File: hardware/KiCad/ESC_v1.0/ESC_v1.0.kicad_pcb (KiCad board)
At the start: 6 copper layers, 56.6 x 43.2 mm, 105 parts, among them J1 Conn_ARM_SWD_TagConnect_TC203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, J3 USB4105-GF-A, Q3 CSD18540Q5B, Q4 CSD18540Q5B, U2 LM5160A, U3 TPS7B92033, U4 STM32G484CEU6, U5 2EDL8024, U8 TPD2EUSB30A, X2 16MHz

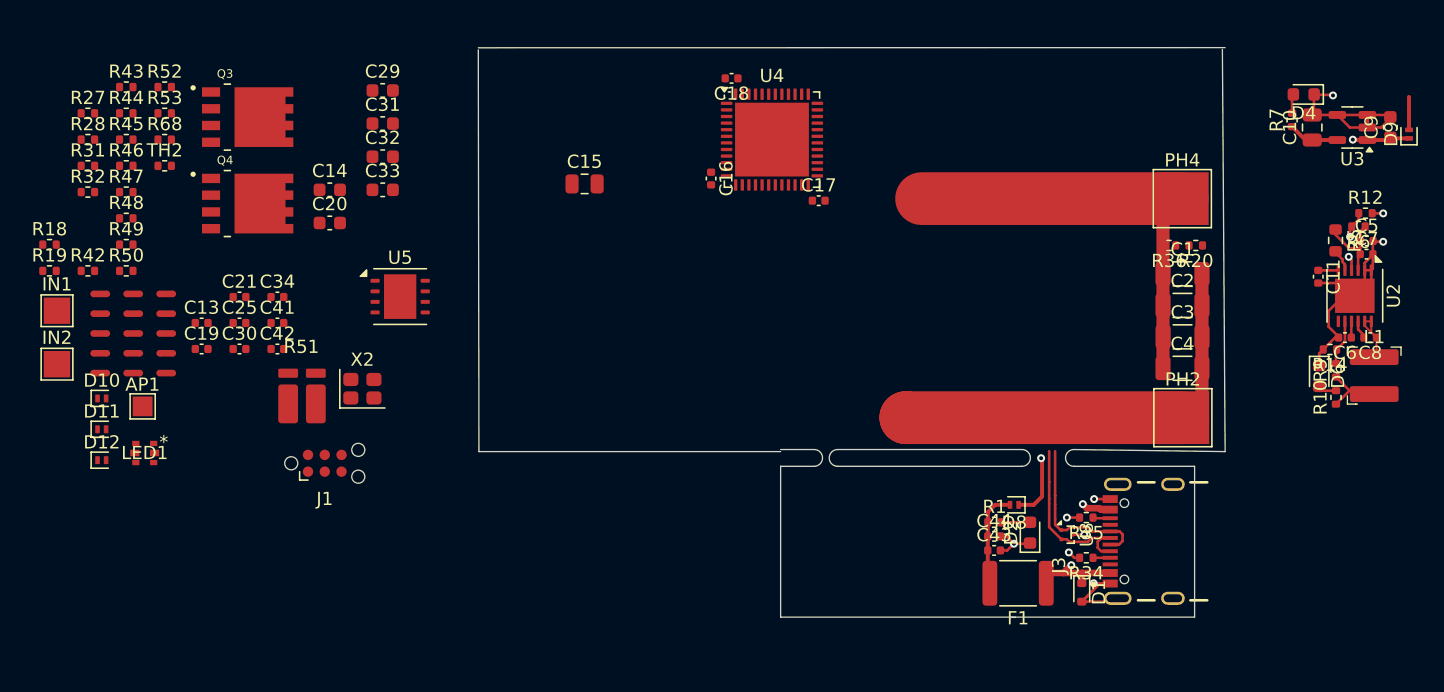
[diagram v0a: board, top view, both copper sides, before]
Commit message: Major board update
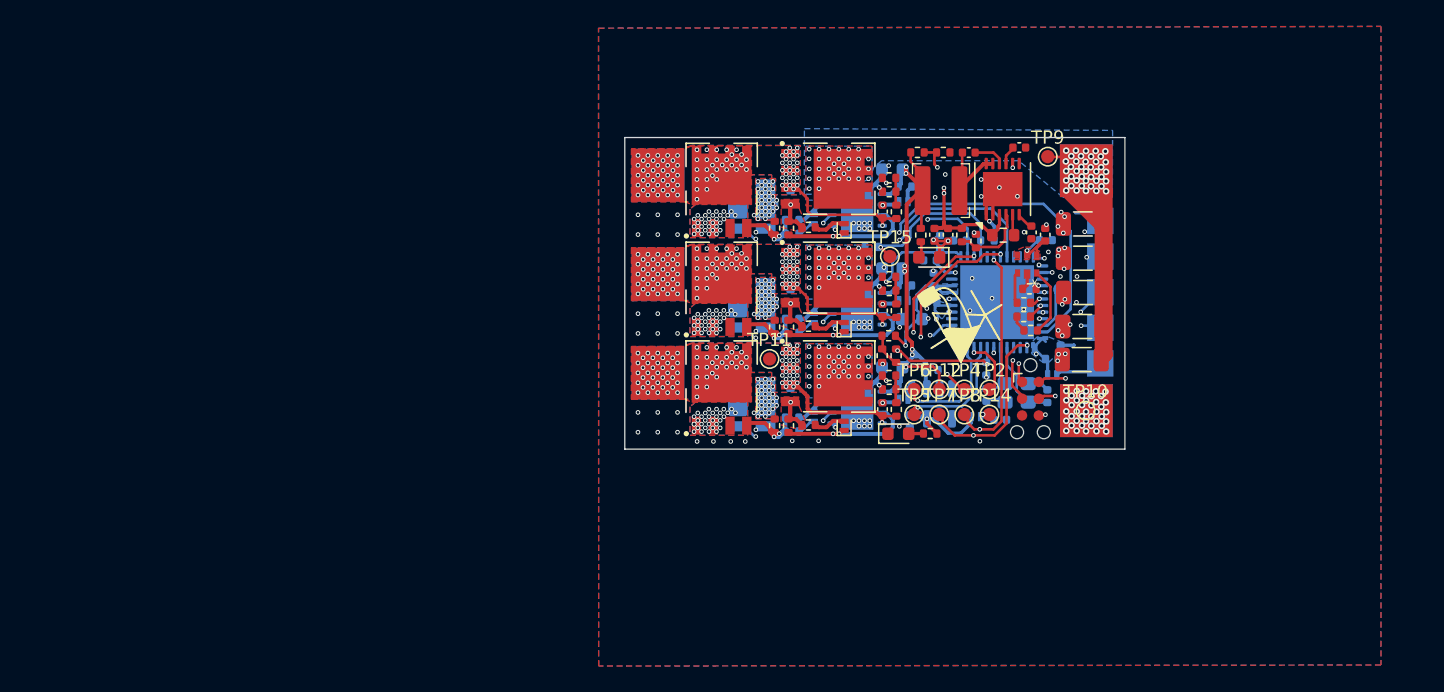
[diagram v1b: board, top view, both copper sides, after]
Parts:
- removed AP1: ActionPad, TestPoint:TestPoint_Pad_1.5x1.5mm
- removed C10: 4.7u, Capacitor_SMD:C_0805_2012Metric
- removed the C14 at (58.5, 45.0)
- removed the C16 at (87.4, 44.1)
- removed the C17 at (95.6, 45.8)
- removed the C4 at (123.2, 58.5)
- removed C41, C42: 10p, Capacitor_SMD:C_0402_1005Metric
- removed C43: 1u, Capacitor_SMD:C_0402_1005Metric
- removed C44: 100n, Capacitor_SMD:C_0402_1005Metric
- removed the C5 at (137.1, 48.8)
- removed C9: 1u, Capacitor_SMD:C_0603_1608Metric
- removed the D1 at (115.5, 75.5)
- removed F1: Polyfuse, Resistor_SMD:R_1812_4532Metric
- removed IN1, IN2: ~, TestPoint:TestPoint_Pad_2.0x2.0mm
- removed NT1, NT10, NT11, NT12, NT13, NT14, NT15, NT2, NT3, NT4, NT5, NT6, NT7, NT8, NT9: NetTie_2, NetTie:NetTie-2_SMD_Pad0.5mm
- removed PH2, PH4: ~, TestPoint:TestPoint_Pad_4.0x4.0mm
- removed the R5 at (134.8, 48.8)
- removed R51: 0.5m, ESC-FootprintLib:Kelvin Shunt 1216 (3038)
- removed R52: 33, Resistor_SMD:R_0402_1005Metric
- removed R53: 10k, Resistor_SMD:R_0402_1005Metric
- removed the R6 at (136.5, 47.7)
- removed R68: 0R, Resistor_SMD:R_0402_1005Metric
- removed TH2: Thermistor_NTC, Resistor_SMD:R_0402_1005Metric
- removed U8: TPD2EUSB30A, Package_TO_SOT_SMD:Texas_DRT-3
- removed X2: 16MHz, Crystal:Crystal_SMD_2520-4Pin_2.5x2.0mm
- added C1: 1u, Capacitor_SMD:C_0402_1005Metric, B.Cu at (102.5, 62.5)
- added C11: 100n, Capacitor_SMD:C_0402_1005Metric, B.Cu at (113.9, 56.3)
- added C12: 1u, Capacitor_SMD:C_0402_1005Metric, F.Cu at (104.4, 48.4)
- added C2: 100n, Capacitor_SMD:C_0402_1005Metric, B.Cu at (104.0, 50.3)
- added C23: 1u, Capacitor_SMD:C_0402_1005Metric, B.Cu at (104.2, 58.6)
- added C24: 100n, Capacitor_SMD:C_0402_1005Metric, B.Cu at (108.3, 58.5)
- added C26: 220n, Capacitor_SMD:C_0402_1005Metric, F.Cu at (100.4, 46.6)
- added C27: 1u, Capacitor_SMD:C_0603_1608Metric, B.Cu at (101.2, 43.4)
- added C28: 100n, Capacitor_SMD:C_0402_1005Metric, B.Cu at (106.3, 48.8)
- added C37: 100n, Capacitor_SMD:C_0402_1005Metric, B.Cu at (112.8, 48.8)
- added C6: 2.2u, Capacitor_SMD:C_1206_3216Metric, F.Cu at (115.6, 55.3)
- added C8: 2.2u, Capacitor_SMD:C_1206_3216Metric, F.Cu at (115.5, 57.8)
- added D13: RB161QS-40T18R, ESC-FootprintLib:Rohm_SMD1006, B.Cu at (95.2, 62.2)
- added D14: RB161QS-40T18R, ESC-FootprintLib:Rohm_SMD1006, B.Cu at (113.3, 59.0)
- added D5: RB161QS-40T18R, ESC-FootprintLib:Rohm_SMD1006, B.Cu at (102.0, 45.9)
- added D6: RB161QS-40T18R, ESC-FootprintLib:Rohm_SMD1006, F.Cu at (97.5, 47.9)
- added D7: RB161QS-40T18R, ESC-FootprintLib:Rohm_SMD1006, B.Cu at (95.2, 47.2)
- added J10: Conn_01x01, TestPoint:TestPoint_Pad_2.0x2.0mm, B.Cu at (116.9, 58.1)
- added J11: JTAG_TC2030, Connector:Tag-Connect_TC2030-IDC-NL_2x03_P1.27mm_Vertical, F.Cu at (111.6, 60.8)
- added J2: Conn_01x01, ESC-FootprintLib:Phase4x4, F.Cu at (115.9, 61.7)
- added J4: Conn_01x01, TestPoint:TestPoint_Pad_2.0x2.0mm, B.Cu at (116.9, 52.7)
- added J5: Conn_01x01, TestPoint:TestPoint_Pad_2.0x2.0mm, B.Cu at (116.9, 47.3)
- added J6: Conn_01x01, TestPoint:TestPoint_Pad_2.0x2.0mm, B.Cu at (116.9, 50.0)
- added J7: Conn_01x01, ESC-FootprintLib:Phase4x4, F.Cu at (83.4, 43.9)
- added J8: Conn_01x01, ESC-FootprintLib:Phase4x4, F.Cu at (83.4, 51.4)
- added J9: Conn_01x01, ESC-FootprintLib:Phase4x4, F.Cu at (83.4, 58.8)
- added Q1: CSD18540Q5B, ESC-FootprintLib:TRANS_CSD18540Q5B, F.Cu at (96.2, 44.1)
- added Q2: CSD18540Q5B, ESC-FootprintLib:TRANS_CSD18540Q5B, F.Cu at (88.2, 45.1)
- added Q5: CSD18540Q5B, ESC-FootprintLib:TRANS_CSD18540Q5B, F.Cu at (96.2, 59.1)
- added Q6: CSD18540Q5B, ESC-FootprintLib:TRANS_CSD18540Q5B, F.Cu at (88.2, 60.1)
- added R11: 100, Resistor_SMD:R_0402_1005Metric, F.Cu at (104.0, 63.4)
- added R13: 33, Resistor_SMD:R_0402_1005Metric, F.Cu at (101.5, 57.5)
- added R14: 100, Resistor_SMD:R_0402_1005Metric, F.Cu at (111.1, 54.6)
- added R15: 100, Resistor_SMD:R_0402_1005Metric, F.Cu at (111.7, 55.6)
- added R16: 100, Resistor_SMD:R_0402_1005Metric, F.Cu at (111.6, 52.5)
- added R17: 100, Resistor_SMD:R_0402_1005Metric, F.Cu at (111.1, 53.5)
- added R2: 10k, Resistor_SMD:R_0402_1005Metric, B.Cu at (108.4, 48.8)
- added R21: 10k, Resistor_SMD:R_0402_1005Metric, B.Cu at (93.5, 45.6)
- added R22: 3.3, Resistor_SMD:R_0402_1005Metric, B.Cu at (93.6, 47.2)
- added R23: 10, Resistor_SMD:R_0402_1005Metric, B.Cu at (93.6, 48.3)
- added R24: 10k, Resistor_SMD:R_0402_1005Metric, F.Cu at (92.3, 47.9)
- added R25: 0.5m, ESC-FootprintLib:Kelvin Shunt 1216 (3038), B.Cu at (90.5, 46.3)
- added R26: 10k, Resistor_SMD:R_0402_1005Metric, F.Cu at (101.5, 46.6)
- added R29: 3.3, Resistor_SMD:R_0402_1005Metric, B.Cu at (102.1, 52.2)
- added R3: 120k, Resistor_SMD:R_0603_1608Metric, F.Cu at (109.6, 48.4)
- added R30: 10, Resistor_SMD:R_0402_1005Metric, F.Cu at (94.8, 55.3)
- added R33: 3.3, Resistor_SMD:R_0402_1005Metric, B.Cu at (93.6, 54.7)
- added R37: 10k, Resistor_SMD:R_0402_1005Metric, F.Cu at (101.5, 54.1)
- added R38: 33, Resistor_SMD:R_0402_1005Metric, F.Cu at (100.9, 51.6)
- added R39: 1k, Resistor_SMD:R_0402_1005Metric, F.Cu at (100.9, 52.6)
- added R4: 200k, Resistor_SMD:R_0402_1005Metric, F.Cu at (106.4, 48.4)
- added R40: 3.3, Resistor_SMD:R_0402_1005Metric, B.Cu at (102.1, 59.7)
- added R41: 10, Resistor_SMD:R_0402_1005Metric, F.Cu at (94.8, 62.8)
- added TH1: Thermistor_NTC, Resistor_SMD:R_0402_1005Metric, F.Cu at (100.4, 57.5)
- added TP1: TestPoint, TestPoint:TestPoint_Pad_D1.0mm, B.Cu at (113.9, 52.5)
- added TP10: TestPoint, TestPoint:TestPoint_Pad_D1.0mm, F.Cu at (115.8, 61.7)
- added TP11: TestPoint, TestPoint:TestPoint_Pad_D1.0mm, F.Cu at (91.9, 57.8)
- added TP12: TestPoint, TestPoint:TestPoint_Pad_D1.0mm, F.Cu at (104.7, 60.1)
- added TP14: TestPoint, TestPoint:TestPoint_Pad_D1.0mm, F.Cu at (108.5, 62.0)
- added TP15: TestPoint, TestPoint:TestPoint_Pad_D1.0mm, F.Cu at (101.0, 50.0)
- added TP2: TestPoint, TestPoint:TestPoint_Pad_D1.0mm, F.Cu at (108.5, 60.1)
- added TP4: TestPoint, TestPoint:TestPoint_Pad_D1.0mm, F.Cu at (106.6, 60.1)
- added TP5: TestPoint, TestPoint:TestPoint_Pad_D1.0mm, F.Cu at (102.8, 62.0)
- added TP6: TestPoint, TestPoint:TestPoint_Pad_D1.0mm, F.Cu at (102.8, 60.1)
- added TP7: TestPoint, TestPoint:TestPoint_Pad_D1.0mm, F.Cu at (104.7, 62.0)
- added TP8: TestPoint, TestPoint:TestPoint_Pad_D1.0mm, F.Cu at (106.6, 62.0)
- added TP9: TestPoint, TestPoint:TestPoint_Pad_D1.0mm, F.Cu at (113.0, 42.5)
- added U1: STM32G484CEU6, ESC-FootprintLib:QFN-48-1EP_7x7mm_P0.5mm_EP5.6x5.6mm, B.Cu at (109.1, 53.5)
- added U6: 2EDL8024, ESC-FootprintLib:2EDL8x2x_PG-VDSON-8-4, B.Cu at (98.5, 61.5)
- added X1: 16MHz, Crystal:Crystal_SMD_2520-4Pin_2.5x2.0mm, B.Cu at (110.6, 60.4)
- C13: value 10n -> 1u
- C15: value 4.7u -> 100n; footprint Capacitor_SMD:C_0805_2012Metric -> Capacitor_SMD:C_0402_1005Metric; moved to B.Cu
- C18: value 100n -> 10n; moved to B.Cu
- C19: value 100n -> 1u; footprint Capacitor_SMD:C_0402_1005Metric -> Capacitor_SMD:C_0603_1608Metric; moved to B.Cu
- C20: value 1u -> 10p; footprint Capacitor_SMD:C_0603_1608Metric -> Capacitor_SMD:C_0402_1005Metric; moved to B.Cu
- C21: value 100n -> 10p; moved to B.Cu
- C29, C32: value 100p -> 220n; footprint Capacitor_SMD:C_0603_1608Metric -> Capacitor_SMD:C_0402_1005Metric
- C30: value 220n -> 1u; footprint Capacitor_SMD:C_0402_1005Metric -> Capacitor_SMD:C_0603_1608Metric; moved to B.Cu
- C31: value 1u -> 100n; footprint Capacitor_SMD:C_0603_1608Metric -> Capacitor_SMD:C_0402_1005Metric; moved to B.Cu
- C33: value 100p -> 1u; moved to B.Cu
- C34, C7, D10, D11, D8, U3, U5: moved to B.Cu
- D2: value KT-0603W -> RB161QS-40T18R; footprint LED_SMD:LED_0603_1608Metric -> ESC-FootprintLib:Rohm_SMD1006; moved to B.Cu
- J1: value Conn_ARM_SWD_TagConnect_TC2030-NL -> Conn_01x01; footprint Connector:Tag-Connect_TC2030-IDC-NL_2x03_P1.27mm_Vertical -> ESC-FootprintLib:Phase4x4
- J3: value USB4105-GF-A -> Conn_01x01; footprint ESC-FootprintLib:GCT_USB4105-GF-A -> TestPoint:TestPoint_Pad_2.0x2.0mm; moved to B.Cu
- R1: value 1k -> 10k; moved to B.Cu
- R12: value 22k -> 10k
- R18: value 100 -> 3.3; moved to B.Cu
- R19: value 100 -> 10
- R20: value 10k -> 3.3
- R27: value 100 -> 33
- R28: value 100 -> 1k
- R32: value 10 -> 10k; moved to B.Cu
- R34: value 5.1k -> 10; moved to B.Cu
- R35: value 5.1k -> 10k
- R36: value 10k -> 0.5m; footprint Resistor_SMD:R_0402_1005Metric -> ESC-FootprintLib:Kelvin Shunt 1216 (3038); moved to B.Cu
- R43: value 33 -> 10k; moved to B.Cu
- R44: value 10k -> 3.3; moved to B.Cu
- R45: value 10k -> 10; moved to B.Cu
- R46: value 1k -> 10k
- R47: value 3.3 -> 0.5m; footprint Resistor_SMD:R_0402_1005Metric -> ESC-FootprintLib:Kelvin Shunt 1216 (3038); moved to B.Cu
- R48: value 10 -> 10k
- R49: value 200k -> 33
- R50: value 10k -> 1k
- R7: value 100 -> 22k
- U4: value STM32G484CEU6 -> 2EDL8024; footprint ESC-FootprintLib:QFN-48-1EP_7x7mm_P0.5mm_EP5.6x5.6mm -> ESC-FootprintLib:2EDL8x2x_PG-VDSON-8-4; moved to B.Cu
- moved LED1 68.4 mm to (111.4, 50.6), turned to -90 degrees
- moved R18 65.0 mm to (102.1, 44.7)
- moved J1 61.8 mm to (115.9, 43.5)
- moved C25 61.4 mm to (112.8, 48.4), turned to 90 degrees
- moved R27 60.9 mm to (100.9, 44.1)
- moved R28 60.9 mm to (100.9, 45.1)
- moved D11 60.8 mm to (102.0, 60.8)
- moved R48 60.1 mm to (101.5, 61.6), turned to 90 degrees
- moved R49 58.6 mm to (100.9, 59.0)
- moved R50 58.5 mm to (100.9, 60.1)
- moved R19 57.6 mm to (94.8, 47.8), turned to 180 degrees
- moved C21 57.1 mm to (108.3, 60.5), turned to -90 degrees
- moved C13 57.0 mm to (105.4, 48.4), turned to -90 degrees
- moved D12 56.3 mm to (97.5, 62.9), turned to 90 degrees
- moved C20 55.9 mm to (112.9, 60.6), turned to 90 degrees
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- renumbered C8 to C14, C6 to C16, C11 to C17, C1 to C3, C2 to C4, C3 to C5, D6 to D1, R10 to R5, R9 to R6, R14 to R8
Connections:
- net Net-(R27-Pad2) renamed /PHASE 1/VS
- net Net-(U2-FB) renamed /FB
- net Net-(U2-SS) renamed /SS
- net Net-(U2-VCC) renamed /VCC
- C13 pad 1: +3V3 -> VBAT
- C15 pad 1: +3V3 -> 3V3
- C18 pad 1: +3V3 -> 3V3
- C19 pad 1: +3V3 -> 3V3
- C20 pad 1: +3V3 -> /HSE_IN
- C21 pad 1: +3V3 -> /HSE_OUT
- C25 pad 1: DEBUG_NRST -> 3V3
- C29 pad 1: /+VSENS1 -> /PHASE 2/HB
- C29 pad 2: GND -> PH2
- C3 pad 2: PGND -> GND
- C30 pad 1: /HB1 -> VBUCK
- C30 pad 2: PH1 -> GND
- C31 pad 1: VBUCK -> /VSENS2
- C32 pad 1: PWM1N -> /PHASE 3/HB
- C32 pad 2: GND -> PH3
- C33 pad 1: PWM1 -> VBUCK
- C34 pad 1: /TSENS1 -> /VSENS3
- C4 pad 2: PGND -> GND
- C5 pad 2: PGND -> GND
- C7 pad 1: VBAT -> GND
- C7 pad 2: GND -> 3V3
- D10 pad 1: /HB1 -> /PHASE 2/LO
- D11 pad 1: /HO -> /PHASE 3/HB
- D12 pad 1: /LO -> /PHASE 3/HO
- D2 pad 1: GND -> 3V3
- D2 pad 2: Net-(D2-A) -> /3V3_LDO
- D8 pad 1: /VIN -> /PHASE 2/HB
- D8 pad 2: +5V -> Net-(D8-A)
- D9 pad 1: /VIN -> /PHASE 2/HO
- D9 pad 2: VBUCK -> Net-(D9-A)
- J1 pad 1: +3V3 -> VBAT
- LED1 pad 1: /LED_R_K -> Net-(LED1-Pad1)
- LED1 pad 2: +3V3 -> 3V3
- LED1 pad 3: /LED_G_K -> Net-(LED1-Pad3)
- LED1 pad 4: +3V3 -> 3V3
- LED1 pad 5: /LED_B_K -> Net-(LED1-Pad5)
- LED1 pad 6: +3V3 -> 3V3
- Q3 pad 2: Net-(Q3-G) -> /PHASE 2/GH
- Q3 pad 3: PH1 -> PH2
- Q4 pad 1: PH1 -> PH2
- Q4 pad 2: Net-(Q4-G) -> /PHASE 2/GL
- Q4 pad 3: /+ISENS1 -> /PHASE 2/LS
- R1 pad 1: +5V -> /VSENSBAT
- R1 pad 2: Net-(D2-A) -> VBAT
- R12 pad 1: Net-(U2-EN/UVLO) -> 3V3
- R12 pad 2: GND -> Net-(R12-Pad2)
- R18 pad 1: RGB_LED_G -> VBUCK
- R18 pad 2: /LED_G_K -> Net-(D5-A)
- R19 pad 1: RGB_LED_B -> Net-(D6-A)
- R19 pad 2: /LED_B_K -> /PHASE 1/GH
- R20 pad 1: GND -> /PHASE 1/HO
- R20 pad 2: /VSENSBAT -> /PHASE 1/GH
- R27 pad 1: /LED_R_K -> /VSENS1
- R28 pad 1: RGB_LED_R -> GND
- R31 pad 1: VBUCK -> /PHASE 2/HO
- R31 pad 2: Net-(D10-A) -> /PHASE 2/GH
- R32 pad 1: Net-(D11-A) -> /PHASE 2/GH
- R32 pad 2: Net-(Q3-G) -> PH2
- R34 pad 1: Net-(J3-CC1) -> Net-(D10-A)
- R34 pad 2: GND -> /PHASE 2/GL
- R35 pad 1: Net-(J3-CC2) -> /PHASE 2/GL
- R36 pad 1: /VSENSBAT -> /ISENS2+
- R36 pad 2: VBAT -> /PHASE 2/LS
- R42 pad 1: /HO -> /PHASE 3/HO
- R42 pad 2: Net-(Q3-G) -> /PHASE 3/GH
- R43 pad 1: /+VSENS1 -> /PHASE 3/GH
- R43 pad 2: Net-(R43-Pad2) -> PH3
- R44 pad 1: Net-(Q3-G) -> /PHASE 3/LO
- R44 pad 2: PH1 -> /PHASE 3/GL
- R45 pad 1: PH1 -> Net-(D13-A)
- R45 pad 2: Net-(R43-Pad2) -> /PHASE 3/GL
- R46 pad 1: GND -> /PHASE 3/GL
- R46 pad 2: Net-(R43-Pad2) -> GND
- R47 pad 1: /LO -> /ISENS3+
- R47 pad 2: Net-(Q4-G) -> /PHASE 3/LS
- R48 pad 1: Net-(D12-A) -> PH3
- R48 pad 2: Net-(Q4-G) -> /PHASE 3/VS
- R49 pad 1: PWM1 -> /VSENS3
- R49 pad 2: GND -> /PHASE 3/VS
- R50 pad 1: Net-(Q4-G) -> GND
- R50 pad 2: GND -> /PHASE 3/VS
- R7 pad 1: +3V3 -> /UVLO
- R7 pad 2: Net-(D4-A) -> GND
- U2 pad 4: Net-(U2-EN/UVLO) -> /UVLO
- U2 pad 5: Net-(U2-RON) -> /RON
- U3 pad 1: /VIN -> VBUCK
- U3 pad 5: +3V3 -> /3V3_LDO
- U4 pad 1: +3V3 -> VBUCK
- U4 pad 2: RGB_LED_B -> /PHASE 1/HB
- U4 pad 3: RGB_LED_G -> /PHASE 1/HO
- U4 pad 4: RGB_LED_R -> PH1
- U4 pad 5: Net-(U4-PF0-OSC_IN) -> /PWM1
- U4 pad 6: Net-(U4-PF1-OSC_OUT) -> /PWM1N
- U4 pad 7: DEBUG_NRST -> GND
- U4 pad 8: /+TSENS1 -> /PHASE 1/LO
- U5 pad 2: /HB1 -> /PHASE 2/HB
- U5 pad 3: /HO -> /PHASE 2/HO
- U5 pad 4: PH1 -> PH2
- U5 pad 5: PWM1 -> /PWM2
- U5 pad 6: PWM1N -> /PWM2N
- U5 pad 8: /LO -> /PHASE 2/LO
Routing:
- net 3V3: track 0.00 -> 54.2 mm, vias 0 -> 7
- net PGND: track 32.5 -> 0.00 mm
- net /PWM1N: track 0.00 -> 31.0 mm, vias 0 -> 2
- net VBUCK: track 8.43 -> 38.6 mm, vias 0 -> 7
- net /PWM3: track 0.00 -> 27.8 mm, vias 0 -> 3
- net /PWM3N: track 0.00 -> 27.0 mm, vias 0 -> 3
- net /ISENS3+: track 0.00 -> 25.6 mm, vias 0 -> 2
- net /ISENS1+: track 0.00 -> 22.8 mm, vias 0 -> 2
- net /ISENS3-: track 0.00 -> 22.3 mm, vias 0 -> 2
- net /ISENS1-: track 0.00 -> 21.2 mm, vias 0 -> 2
- net VBAT: track 40.2 -> 59.6 mm, vias 0 -> 142
- net /ISENS2+: track 0.00 -> 18.2 mm, vias 0 -> 2
- net /PWM1: track 0.00 -> 18.2 mm, vias 0 -> 2
- net /PWM2: track 0.00 -> 17.9 mm, vias 0 -> 3
- net /PWM2N: track 0.00 -> 16.7 mm, vias 0 -> 3
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- added copper zone on F.Cu, net /PHASE 1/GH
- added copper zone on B.Cu, net /PHASE 1/LS
- added copper zone on F.Cu, net /PHASE 1/LS
- added copper zone on F.Cu, net /PHASE 2/GH
- added copper zone on B.Cu, net /PHASE 2/LS
- added copper zone on F.Cu, net /PHASE 2/LS
- added copper zone on F.Cu, net /PHASE 3/GH
- added copper zone on B.Cu, net /PHASE 3/LS
- added copper zone on F.Cu, net /PHASE 3/LS
- added copper zone on B.Cu, net /VSENS3
- added copper zone on B.Cu, net 3V3
- added copper zone on F.Cu, net 3V3
- added copper zone on B.Cu, net GND
- added copper zone on F.Cu, net GND
- added copper zone on In2.Cu, net GND
- added copper zone on In3.Cu, net GND
- added copper zone on In4.Cu, net GND
- added copper zone on B.Cu, net PH1
- added copper zone on F.Cu, net PH1
- added copper zone on B.Cu, net PH2
- added copper zone on F.Cu, net PH2
- added copper zone on B.Cu, net PH3
- added copper zone on F.Cu, net PH3
- added copper zone on B.Cu, net VBAT
- added copper zone on F.Cu, net VBAT
- added copper zone on In2.Cu, net VBAT
- added copper zone on In3.Cu, net VBAT
- removed copper zone on In1.Cu, net PGND
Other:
- board size 56.6 x 43.2 mm -> 37.9 x 23.6 mm
- board text added: "3V3"
- board text added: "GND"
- board text added: "Kururugi"
- board text added: "RX"
- board text added: "SB"
- board text added: "TH"
- board text added: "TX"
- board text added: "v1.0"

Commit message: Major Kicad Update
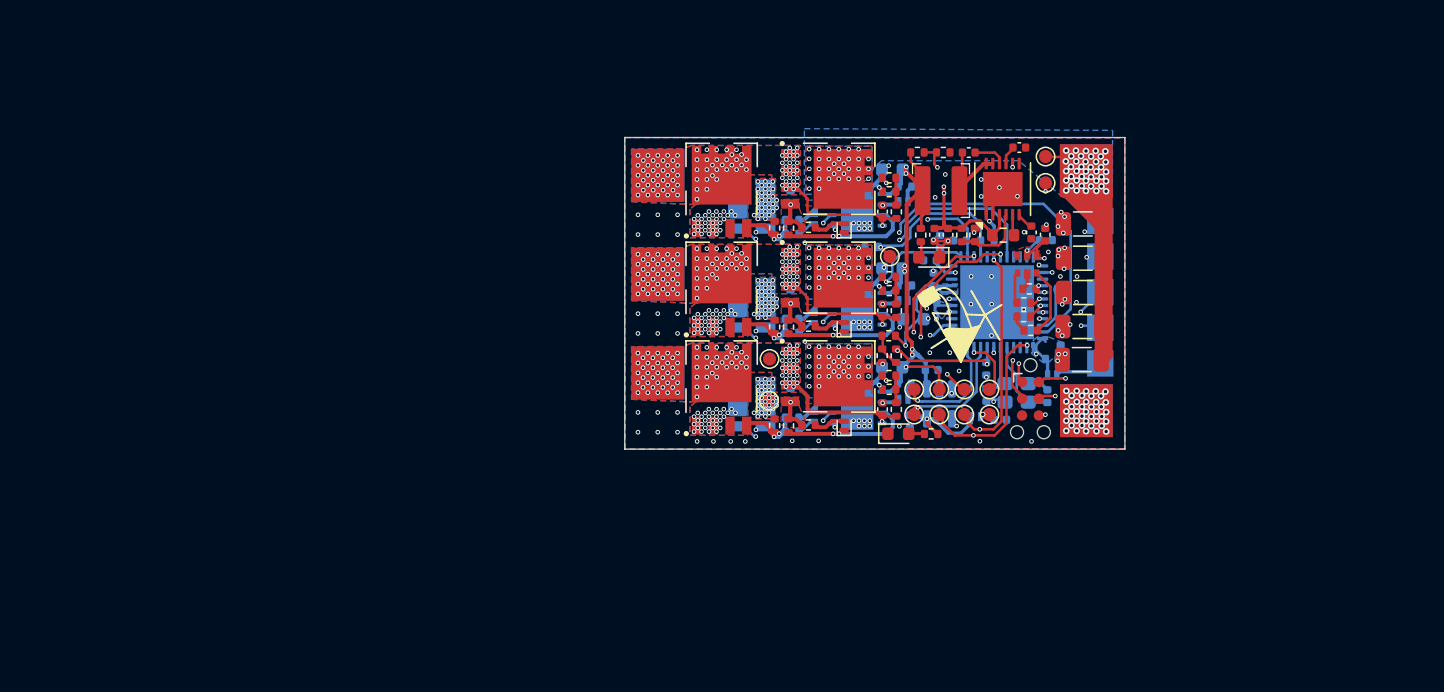
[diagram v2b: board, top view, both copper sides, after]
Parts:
- added TP13: TestPoint, ESC-FootprintLib:TestPoint_Pad_D1.0mm, F.Cu at (91.8, 60.9)
- J10, J3, J4, J5, J6: footprint TestPoint:TestPoint_Pad_2.0x2.0mm -> ESC-FootprintLib:TestPoint_Pad_2.0x2.0mm
- J11: footprint Connector:Tag-Connect_TC2030-IDC-NL_2x03_P1.27mm_Vertical -> ESC-FootprintLib:Tag-Connect_TC2030-IDC-NL_2x03_P1.27mm_Vertical
- TP1, TP10, TP11, TP12, TP14, TP15, TP2, TP4, TP5, TP6, TP7, TP8, TP9: footprint TestPoint:TestPoint_Pad_D1.0mm -> ESC-FootprintLib:TestPoint_Pad_D1.0mm
- moved TP10 17.5 mm to (112.8, 44.4)
- moved R7 0.47 mm to (107.4, 48.4)
- moved TP9 0.16 mm to (112.8, 42.4)
- moved C19 0.12 mm to (102.8, 54.8)
- moved R11 0.08 mm to (104.1, 63.5)
- moved R40 0.06 mm to (102.1, 59.6)
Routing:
- net VBAT: track 59.6 -> 56.1 mm
- net /THROTTLE_CMD: track 8.08 -> 6.78 mm
- net 3V3: track 54.2 -> 53.0 mm
- net VBUCK: track 38.6 -> 39.5 mm
- net GND: track 37.8 -> 38.4 mm, vias 226 -> 238
- net /PHASE 3/LS: vias 32 -> 31
